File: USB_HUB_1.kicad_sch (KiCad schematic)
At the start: 30 parts, among them U11 VL822-QFN76, U12 W25Q32JVZPIQ, Y4 25Mhz

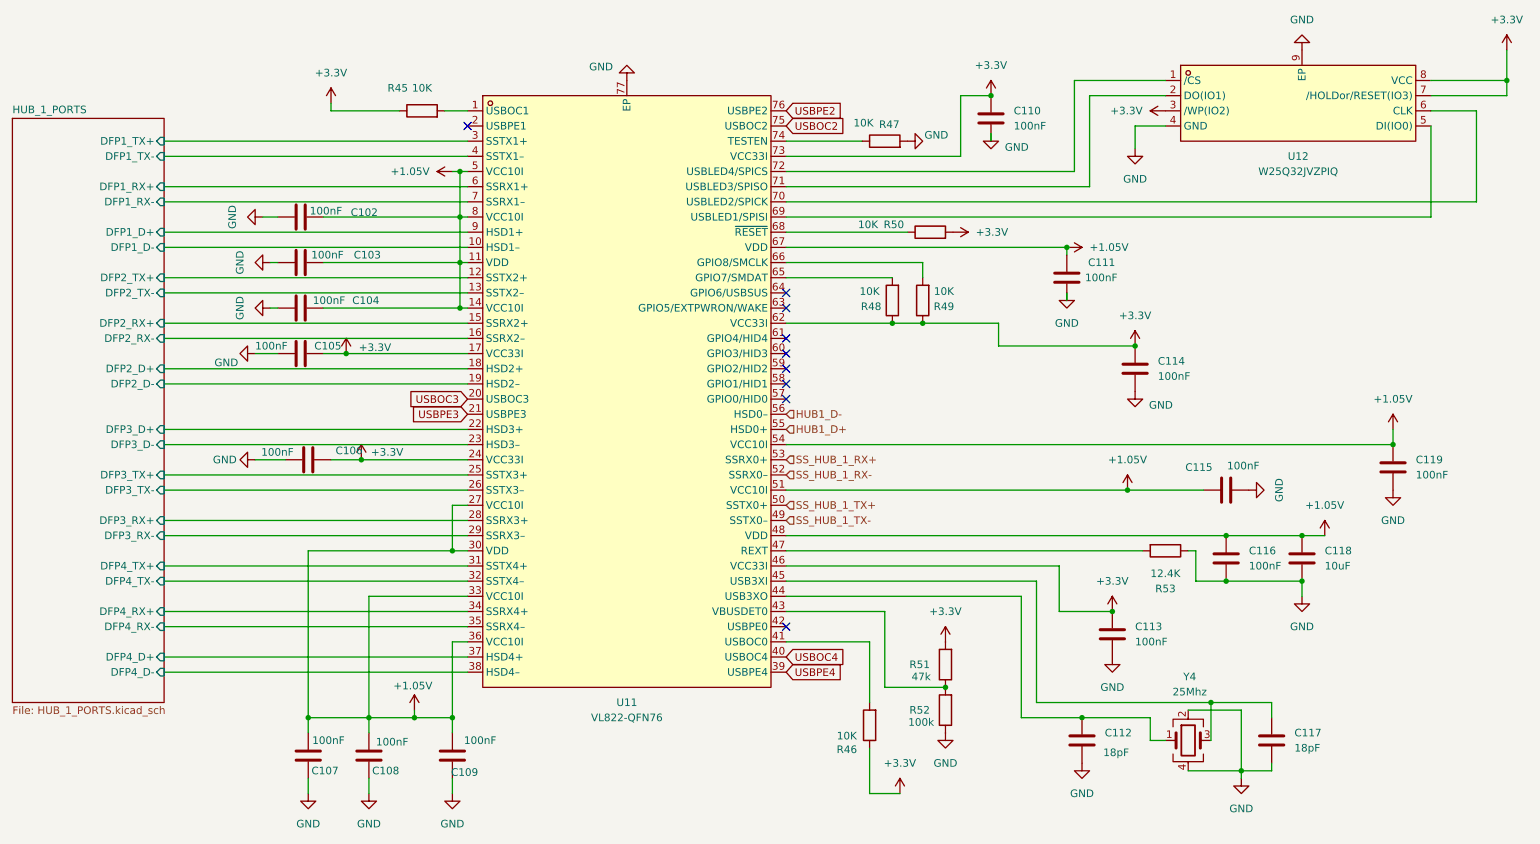
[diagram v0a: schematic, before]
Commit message: .
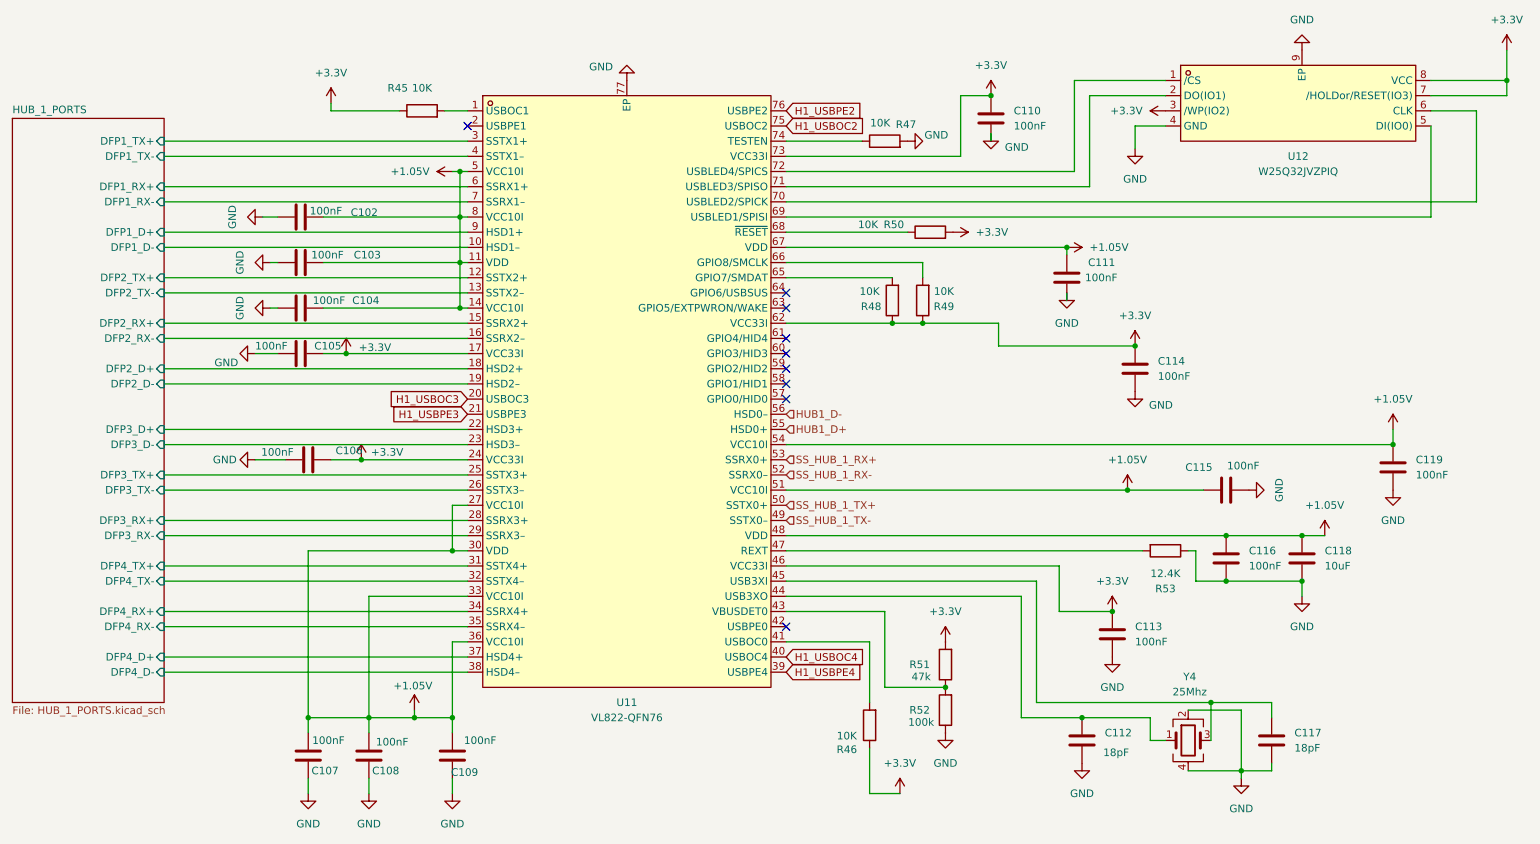
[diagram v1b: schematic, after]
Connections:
- net USBOC2 renamed H1_USBOC2
- net USBOC3 renamed H1_USBOC3
- net USBOC4 renamed H1_USBOC4
- net USBPE2 renamed H1_USBPE2
- net USBPE3 renamed H1_USBPE3
- net USBPE4 renamed H1_USBPE4
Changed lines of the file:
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@@
 		)
 	)
-	(global_label "USBPE3"
+	(global_label "H1_USBPE3"
 		(shape input)
 		(at 104.14 91.44 180)
@@
 		)
 		(property "Intersheetrefs" "${INTERSHEET_REFS}"
-			(at 93.7163 91.44 0)
+			(at 90.2087 91.44 0)
 			(effects
 				(font
@@
 		)
 	)
-	(global_label "USBPE2"
+	(global_label "H1_USBPE2"
 		(shape input)
 		(at 157.48 40.64 0)
@@
 		)
 		(property "Intersheetrefs" "${INTERSHEET_REFS}"
-			(at 167.9037 40.64 0)
+			(at 171.4113 40.64 0)
 			(effects
 				(font
@@
 		)
 	)
-	(global_label "USBOC4"
+	(global_label "H1_USBOC4"
 		(shape input)
 		(at 157.48 132.08 0)
@@
 		)
 		(property "Intersheetrefs" "${INTERSHEET_REFS}"
-			(at 168.0852 132.08 0)
+			(at 171.5928 132.08 0)
 			(effects
 				(font
@@
 		)
 	)
-	(global_label "USBPE4"
+	(global_label "H1_USBPE4"
 		(shape input)
 		(at 157.48 134.62 0)
@@
 		)
 		(property "Intersheetrefs" "${INTERSHEET_REFS}"
-			(at 167.9037 134.62 0)
+			(at 171.4113 134.62 0)
 			(effects
 				(font
@@
 		)
 	)
-	(global_label "USBOC2"
+	(global_label "H1_USBOC2"
 		(shape input)
 		(at 157.48 43.18 0)
@@
 		)
 		(property "Intersheetrefs" "${INTERSHEET_REFS}"
-			(at 168.0852 43.18 0)
+			(at 171.5928 43.18 0)
 			(effects
 				(font
@@
 		)
 	)
-	(global_label "USBOC3"
+	(global_label "H1_USBOC3"
 		(shape input)
 		(at 104.14 88.9 180)
@@
 		)
 		(property "Intersheetrefs" "${INTERSHEET_REFS}"
-			(at 93.5348 88.9 0)
+			(at 90.0272 88.9 0)
 			(effects
 				(font
@@
 		(dnp no)
 		(property "Reference" "R47"
-			(at 174.752 42.926 90)
+			(at 177.546 42.926 90)
 			(effects
 				(font
@@
 		)
 		(property "Value" "10K"
-			(at 170.434 42.672 90)
-			(effects
-				(font
+			(at 173.228 42.672 90)
+			(effects
+				(font
